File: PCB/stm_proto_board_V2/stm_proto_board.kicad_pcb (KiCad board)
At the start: 2 copper layers, 137.2 x 81.3 mm, 48 parts, among them J1 Conn_01x08, J10 Conn_01x02, J11 Conn_01x04, J12 Conn_01x04, J13 Conn_01x04, J14 Conn_01x08, J15 Conn_01x02, J16 Conn_01x03, J17 Conn_01x02, J18 Conn_01x03, J19 Conn_01x04, J2 Conn_01x04, J3 DB9_Female, J4 Conn_01x02, J5 Conn_01x02, J6 Conn_01x02, J7 Conn_01x04, J8 Conn_01x04, J9 Conn_01x04, SW1 SW_Push, SW2 SW_Push, SW3 SW_Push, SW4 SW_Push, U1 YAAJ_BluePill_Part_Like, U2 MCP2551-I-P, U4 LTV-814, U5 L7805, U6 4N25, U7 4N25, U8 4N25, U9 4N25

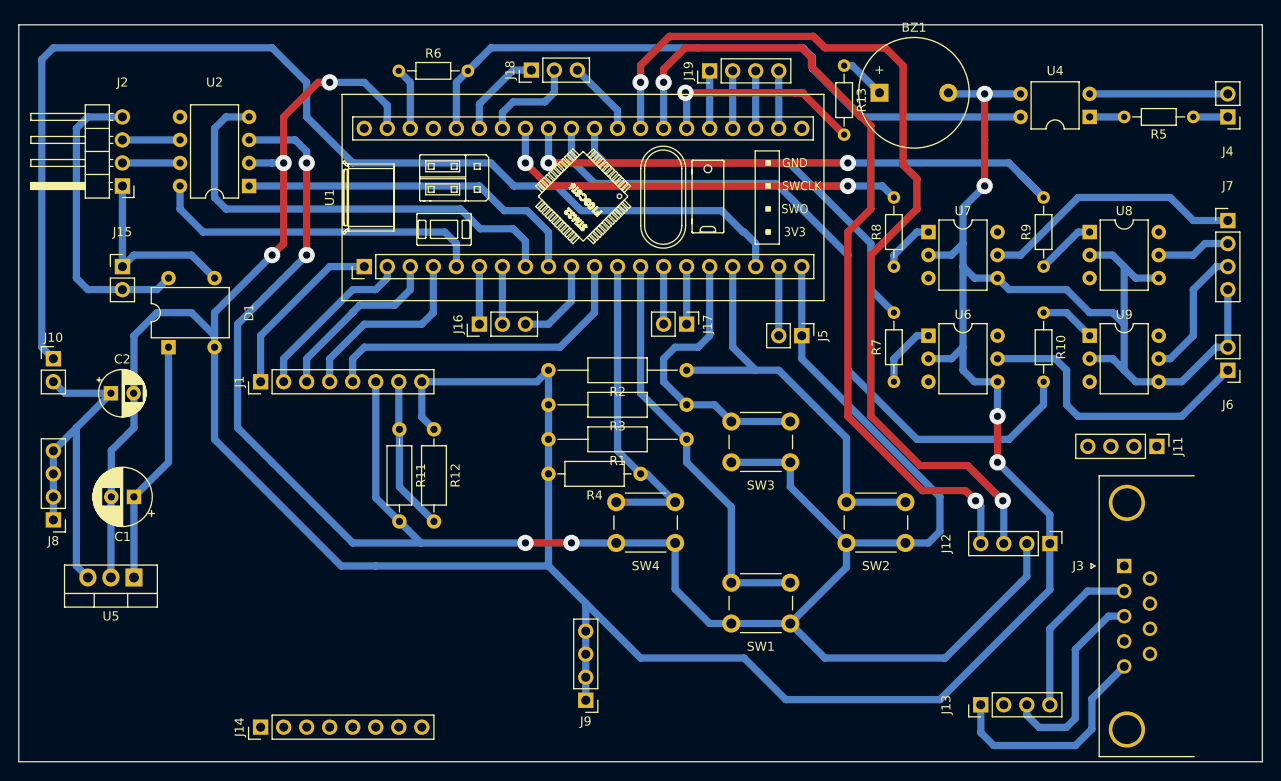
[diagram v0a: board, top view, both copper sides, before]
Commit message: update PCB
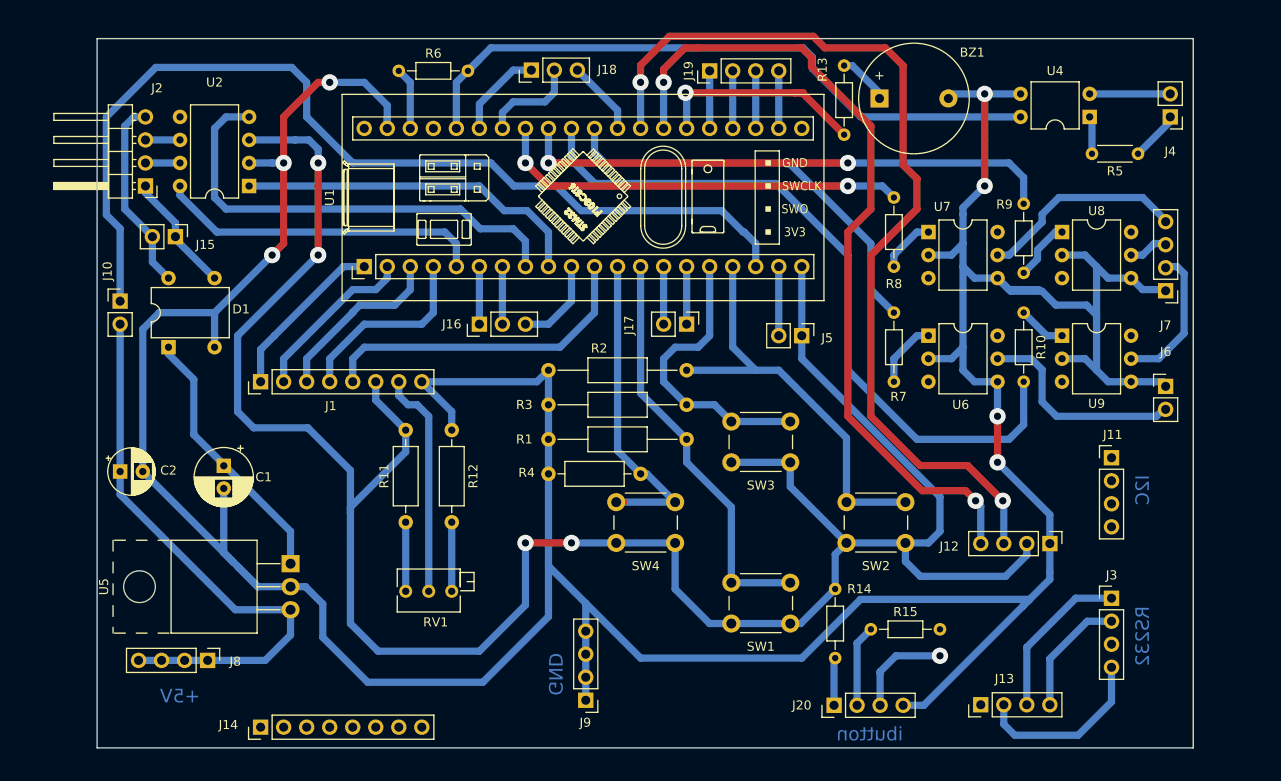
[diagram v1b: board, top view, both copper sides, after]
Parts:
- added J20: Conn_01x04, Connector_PinHeader_2.54mm:PinHeader_1x04_P2.54mm_Vertical, F.Cu at (167.4, 138.6)
- added R14: 330, Resistor_THT:R_Axial_DIN0204_L3.6mm_D1.6mm_P7.62mm_Horizontal, F.Cu at (167.5, 133.3)
- added R15: 330, Resistor_THT:R_Axial_DIN0204_L3.6mm_D1.6mm_P7.62mm_Horizontal, F.Cu at (171.4, 130.2)
- added RV1: R_POT, Potentiometer_THT:Potentiometer_Bourns_3266Z_Horizontal, F.Cu at (120.1, 126.0)
- J3: value DB9_Female -> Conn_01x04; footprint Connector_Dsub:DSUB-9_Female_Horizontal_P2.77x2.84mm_EdgePinOffset4.94mm_Housed_MountingHolesOffset7.48mm -> Connector_PinHeader_2.54mm:PinHeader_1x04_P2.54mm_Vertical
- R5: footprint Resistor_THT:R_Axial_DIN0204_L3.6mm_D1.6mm_P7.62mm_Horizontal -> Resistor_THT:R_Axial_DIN0204_L3.6mm_D1.6mm_P5.08mm_Horizontal
- U5: footprint Package_TO_SOT_THT:TO-220-3_Vertical -> Package_TO_SOT_THT:TO-220-3_Horizontal_TabUp
- moved J8 23.0 mm to (98.3, 133.6), turned to 270 degrees
- moved U5 17.3 mm to (107.4, 122.9), turned to 270 degrees
- moved C1 10.5 mm to (100.1, 112.1), turned to 270 degrees
- moved J7 10.3 mm to (204.0, 92.8), turned to 180 degrees
- moved R11 10.3 mm to (120.1, 118.4), turned to 90 degrees
- moved J10 9.73 mm to (88.6, 94.0)
- moved C2 8.70 mm to (88.6, 112.8)
- moved R5 7.33 mm to (200.9, 77.7)
- moved J6 7.08 mm to (204.0, 103.4), turned to 0 degrees
- moved J15 6.71 mm to (94.7, 86.9), turned to 270 degrees
- moved J4 6.35 mm to (204.5, 73.7)
- moved J11 5.16 mm to (198.0, 111.3), turned to 0 degrees
- moved J3 3.82 mm to (198.0, 126.7), turned to 0 degrees
- moved U8 3.05 mm to (192.5, 86.4)
- moved U9 3.05 mm to (192.5, 97.8)
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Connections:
- net Net-(J13-Pad4) renamed /RS232_TX
- J13 pad 1: Net-(J13-Pad1) -> /RS232_GND
- J13 pad 2: Net-(J13-Pad2) -> /GND_232
- J13 pad 3: Net-(J13-Pad3) -> /RS232_RX
- J3 pad 1: Net-(J3-Pad1) -> /RS232_RX
- J3 pad 3: Net-(J13-Pad3) -> Net-(J3-Pad3)
- J3 pad 4: Net-(J3-Pad4) -> /GND_232
- J6 pad 1: OUT_W -> GND
- J6 pad 2: GND -> OUT_W
- J7 pad 1: OUT_R -> GND
- J7 pad 2: OUT_G -> OUT_B
- J7 pad 3: OUT_B -> OUT_G
- J7 pad 4: GND -> OUT_R
- R11 pad 1: /LIGHT -> Net-(R11-Pad1)
- R12 pad 2: /LIGHT -> Net-(R12-Pad2)
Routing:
- net GND: track 403.3 -> 433.6 mm, vias 7 -> 8
- net Net-(J13-Pad1): track 25.1 -> 0.00 mm
- net +5V: track 40.5 -> 63.6 mm
- net Net-(J13-Pad3): track 22.0 -> 0.00 mm
- net /GND_232: track 0.00 -> 19.9 mm
- net Net-(J10-Pad1): track 126.5 -> 107.7 mm
- net /RS232_RX: track 0.00 -> 17.9 mm
- net /Valt2: track 33.3 -> 21.5 mm
- net Net-(J20-Pad2): track 0.00 -> 9.01 mm
- net OUT_W: track 32.4 -> 23.7 mm
- net /LIGHT: track 17.0 -> 25.1 mm
- net Net-(R12-Pad2): track 0.00 -> 7.62 mm
- net Net-(R11-Pad1): track 0.00 -> 7.62 mm
- net /Valt1: track 20.6 -> 13.3 mm
- net +3V3: track 244.1 -> 251.3 mm
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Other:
- board size 137.2 x 81.3 mm -> 120.9 x 78.2 mm
- board text added: "+5V"
- board text added: "GND"
- board text added: "I2C"
- board text added: "RS232"
- board text added: "ibutton"
